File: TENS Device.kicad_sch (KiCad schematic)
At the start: 3 parts, among them SW1 SW_Push

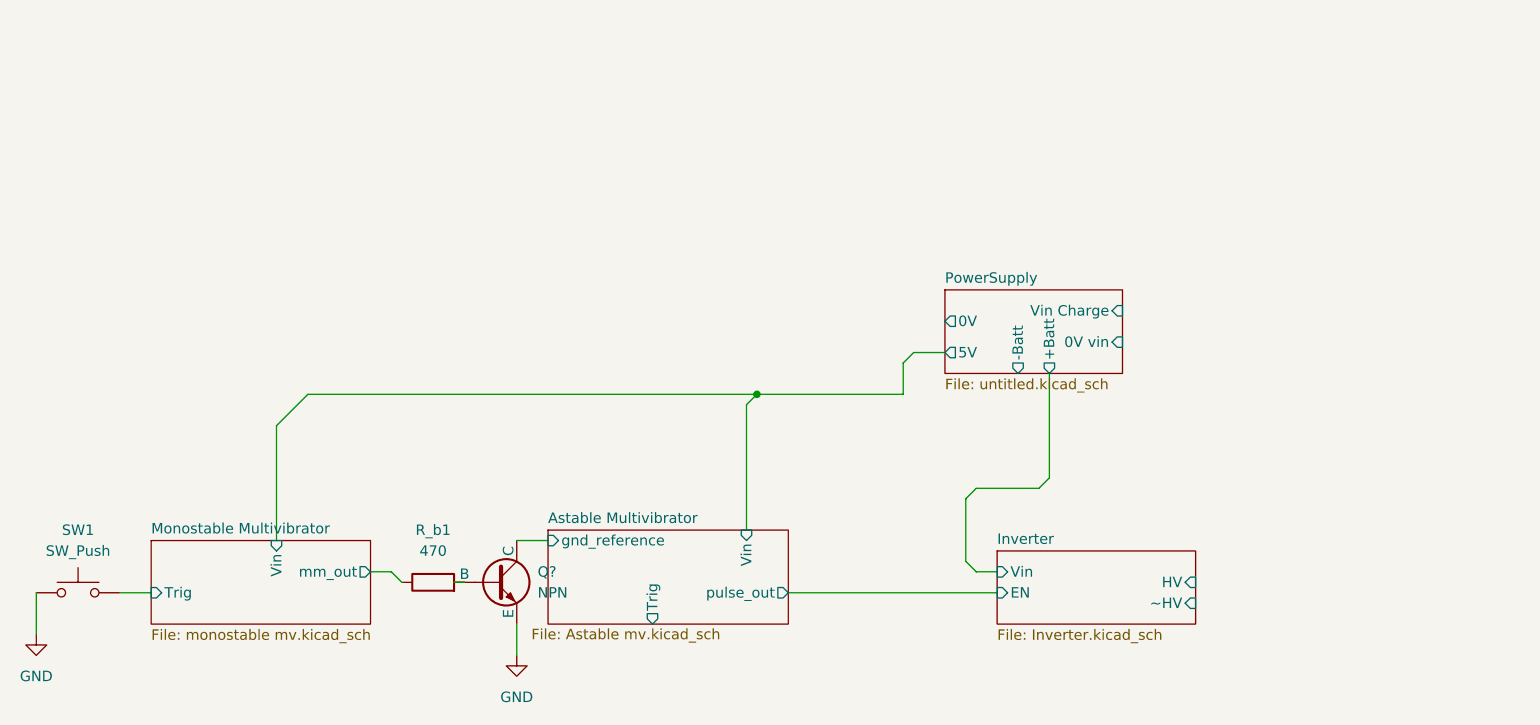
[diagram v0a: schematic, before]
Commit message: update
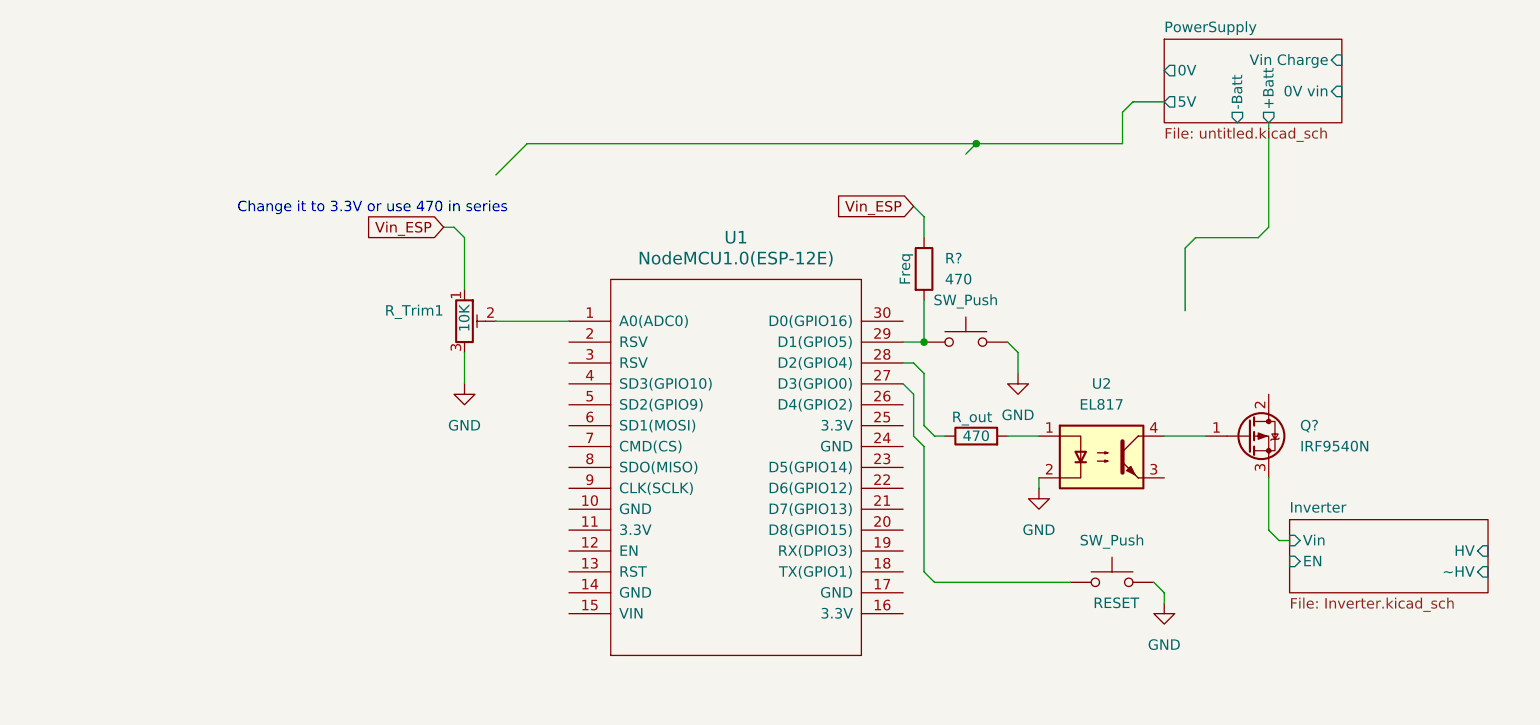
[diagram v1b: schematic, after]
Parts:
- removed Q?: NPN, symbol Simulation_SPICE:NPN
- removed R_b1: 470, symbol Device:R
- removed SW1: SW_Push, symbol Switch:SW_Push
- added Freq, RESET: SW_Push, symbol Switch:SW_Push
- added Q?: IRF9540N, Package_TO_SOT_THT:TO-220-3_Vertical, symbol Transistor_FET:IRF9540N
- added R?, R_out: 470, symbol Device:R
- added R_Trim1: 10K, symbol Device:R_Potentiometer_Trim
- added U1: NodeMCU1.0(ESP-12E), symbol ESP8266:NodeMCU1.0(ESP-12E)
- added U2: EL817, Package_DIP:DIP-4_W7.62mm, symbol Isolator:EL817
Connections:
- net GND: now also Freq.2, RESET.2, R_Trim1.3, U2.2
- net Inverter/Vin: now also Q?.3 (S)
- new net: R_Trim1.2, U1.1 (A0(ADC0))
- new net: RESET.1, U1.27 (D3(GPIO0))
- new net: R_out.1, U1.28 (D2(GPIO4))
- new net: Freq.1, R?.2, U1.29 (D1(GPIO5))
- new net: R_out.2, U2.1
- new net: Q?.1 (G), U2.4
- new net Vin_ESP: R?.1, R_Trim1.1
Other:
- removed sheet Astable Multivibrator
- removed sheet Monostable Multivibrator
- note added: "Change it to 3.3V or use 470 in series"
